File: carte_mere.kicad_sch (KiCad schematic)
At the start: 22 parts, among them J10 Conn_01x02_Pin, J11 Conn_01x02_Pin, J12 Conn_01x02_Pin, J13 Conn_01x02_Pin, J14 Conn_01x02, J20 Conn_01x04, J23 Conn_01x02

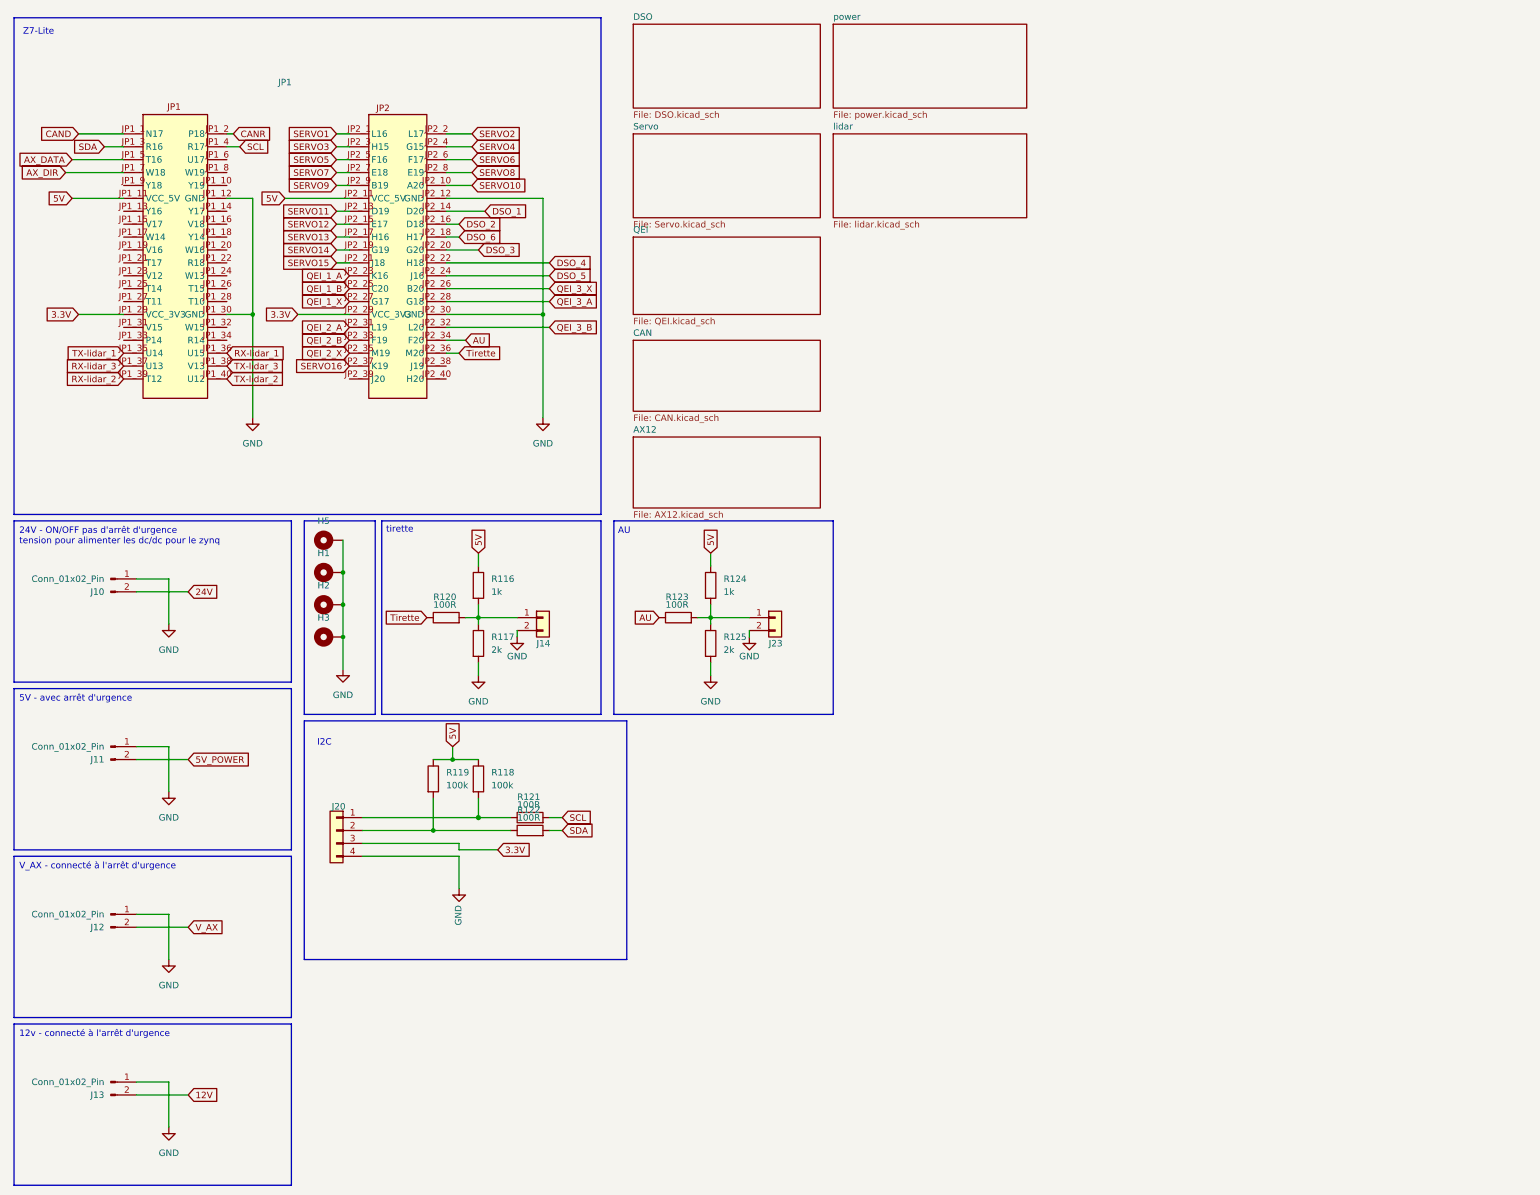
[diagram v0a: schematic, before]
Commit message: clean
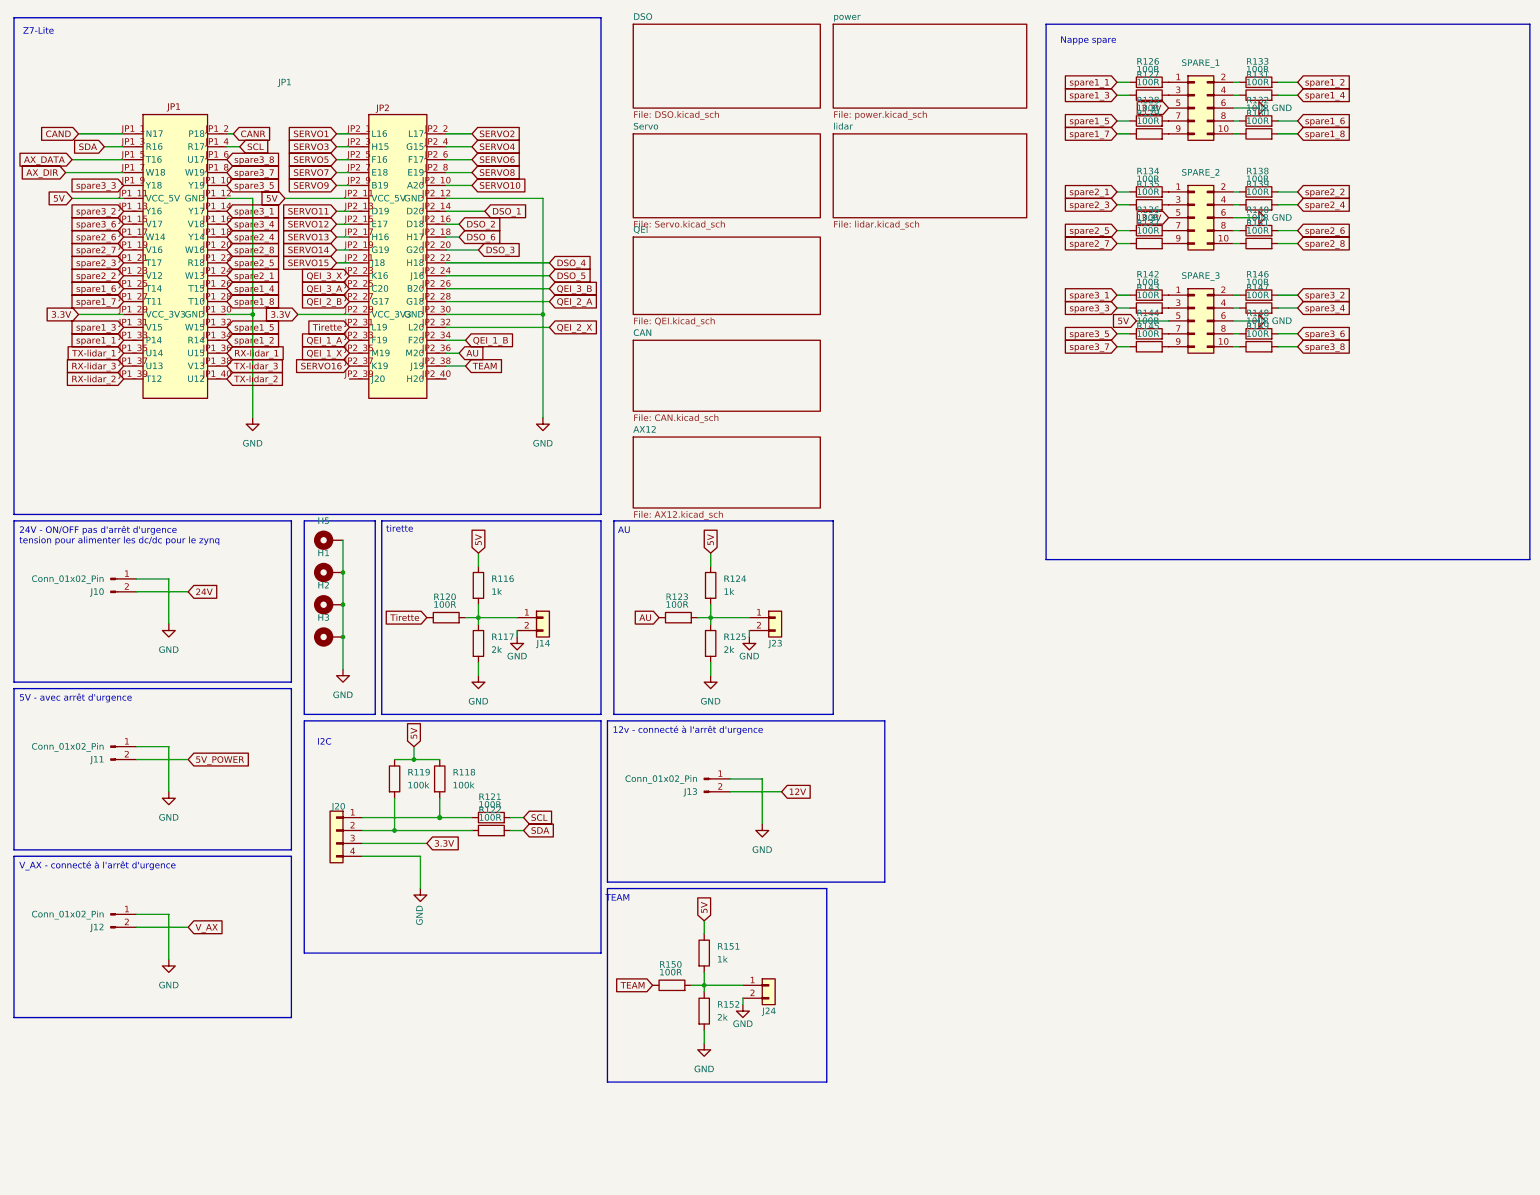
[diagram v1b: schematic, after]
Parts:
- added J24: Conn_01x02, Connector_Molex:Molex_KK-254_AE-6410-02A_1x02_P2.54mm_Vertical, symbol Connector_Generic:Conn_01x02
- added R126, R127, R128, R129, R130, R131, R132, R133, R134, R135, R136, R137, R138, R139, R140, R141, R142, R143, R144, R145, R146, R147, R148, R149, R150: 100R, Capacitor_SMD:C_0402_1005Metric, symbol Device:R
- added R151: 1k, Capacitor_SMD:C_0402_1005Metric, symbol Device:R
- added R152: 2k, Capacitor_SMD:C_0402_1005Metric, symbol Device:R
- added SPARE_1, SPARE_2, SPARE_3: Conn_02x05_Odd_Even, Connector_PinSocket_2.54mm:PinSocket_2x05_P2.54mm_Vertical, symbol Connector_Generic:Conn_02x05_Odd_Even
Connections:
- net 3.3V: now also SPARE_1.5 (Pin_5), SPARE_2.5 (Pin_5)
- net 5V: now also R151.1, SPARE_3.5 (Pin_5)
- net AU: now also JP1.JP2_36 (M20); no longer JP1.JP2_34 (F20)
- net GND: now also J24.2 (Pin_2), R152.2, SPARE_1.6 (Pin_6), SPARE_2.6 (Pin_6), SPARE_3.6 (Pin_6)
- net QEI_1_A: now also JP1.JP2_33 (F19); no longer JP1.JP2_23 (K16)
- net QEI_1_B: now also JP1.JP2_34 (F20); no longer JP1.JP2_25 (C20)
- net QEI_1_X: now also JP1.JP2_35 (M19); no longer JP1.JP2_27 (G17)
- net QEI_2_A: now also JP1.JP2_28 (G18); no longer JP1.JP2_31 (L19)
- net QEI_2_B: now also JP1.JP2_27 (G17); no longer JP1.JP2_33 (F19)
- net QEI_2_X: now also JP1.JP2_32 (L20); no longer JP1.JP2_35 (M19)
- net QEI_3_A: now also JP1.JP2_25 (C20); no longer JP1.JP2_28 (G18)
- net QEI_3_B: now also JP1.JP2_26 (B20); no longer JP1.JP2_32 (L20)
- net QEI_3_X: now also JP1.JP2_23 (K16); no longer JP1.JP2_26 (B20)
- net Tirette: now also JP1.JP2_31 (L19); no longer JP1.JP2_36 (M20)
- net spare3_5: now reaches JP1.JP1_10 (Y19)
- net spare3_5: now also R144.1
- net spare3_2: now reaches JP1.JP1_13 (Y16)
- net spare3_2: now also R146.2
- net spare3_1: now reaches JP1.JP1_14 (Y17)
- net spare3_1: now also R142.1
- net spare3_6: now reaches JP1.JP1_15 (V17)
- net spare3_6: now also R148.2
- net spare3_4: now reaches JP1.JP1_16 (V18)
- net spare3_4: now also R147.2
- net spare2_6: now reaches JP1.JP1_17 (W14)
- net spare2_6: now also R140.2
- net spare2_4: now reaches JP1.JP1_18 (Y14)
- net spare2_4: now also R139.2
- net spare2_7: now reaches JP1.JP1_19 (V16)
- net spare2_7: now also R137.1
- net spare2_8: now reaches JP1.JP1_20 (W16)
- net spare2_8: now also R141.2
- net spare2_3: now reaches JP1.JP1_21 (T17)
- net spare2_3: now also R135.1
- net spare2_5: now reaches JP1.JP1_22 (R18)
- net spare2_5: now also R136.1
- net spare2_2: now reaches JP1.JP1_23 (V12)
- net spare2_2: now also R138.2
- net spare2_1: now reaches JP1.JP1_24 (W13)
- net spare2_1: now also R134.1
- net spare1_6: now reaches JP1.JP1_25 (T14)
- net spare1_6: now also R132.2
- net spare1_4: now reaches JP1.JP1_26 (T15)
- net spare1_4: now also R131.2
- net spare1_7: now reaches JP1.JP1_27 (T11)
- net spare1_7: now also R129.1
- net spare1_8: now reaches JP1.JP1_28 (T10)
- net spare1_8: now also R130.2
- net spare1_3: now reaches JP1.JP1_31 (V15)
- net spare1_3: now also R127.1
- net spare1_5: now reaches JP1.JP1_32 (W15)
- net spare1_5: now also R128.1
- net spare1_1: now reaches JP1.JP1_33 (P14)
- net spare1_1: now also R126.1
- net spare1_2: now reaches JP1.JP1_34 (R14)
- net spare1_2: now also R133.2
- net spare3_8: now reaches JP1.JP1_6 (U17)
- net spare3_8: now also R149.2
- net spare3_7: now reaches JP1.JP1_8 (W19)
- net spare3_7: now also R145.1
- net spare3_3: now reaches JP1.JP1_9 (Y18)
- net spare3_3: now also R143.1
- net TEAM: now reaches JP1.JP2_38 (J19)
- net TEAM: now also R150.1
- new net: R140.1, SPARE_2.8 (Pin_8)
- new net: R149.1, SPARE_3.10 (Pin_10)
- new net: R127.2, SPARE_1.3 (Pin_3)
- new net: R129.2, SPARE_1.9 (Pin_9)
- new net: R141.1, SPARE_2.10 (Pin_10)
- new net: J24.1 (Pin_1), R150.2, R151.2, R152.1
- new net: R131.1, SPARE_1.4 (Pin_4)
- new net: R139.1, SPARE_2.4 (Pin_4)
- new net: R135.2, SPARE_2.3 (Pin_3)
- new net: R133.1, SPARE_1.2 (Pin_2)
- new net: R130.1, SPARE_1.10 (Pin_10)
- new net: R126.2, SPARE_1.1 (Pin_1)
- new net: R128.2, SPARE_1.7 (Pin_7)
- new net: R132.1, SPARE_1.8 (Pin_8)
- new net: R134.2, SPARE_2.1 (Pin_1)
- new net: R138.1, SPARE_2.2 (Pin_2)
- new net: R136.2, SPARE_2.7 (Pin_7)
- new net: R137.2, SPARE_2.9 (Pin_9)
- new net: R142.2, SPARE_3.1 (Pin_1)
- new net: R146.1, SPARE_3.2 (Pin_2)
- new net: R143.2, SPARE_3.3 (Pin_3)
- new net: R147.1, SPARE_3.4 (Pin_4)
- new net: R144.2, SPARE_3.7 (Pin_7)
- new net: R148.1, SPARE_3.8 (Pin_8)
- new net: R145.2, SPARE_3.9 (Pin_9)
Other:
- note added: "Nappe spare"
- note added: "TEAM"
- moved on the sheet: J13, R118, R119, R121, R122
